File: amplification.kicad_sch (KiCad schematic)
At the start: 34 parts, among them Q1 PNP, Q10 PNP, Q11 NPN, Q12 NPN, Q13 NPN, Q14 PNP, Q15 NPN, Q16 PNP, Q2 PNP, Q3 NPN, Q4 PNP, Q5 NPN, Q6 PNP, Q7 NPN, Q8 NPN, Q9 PNP

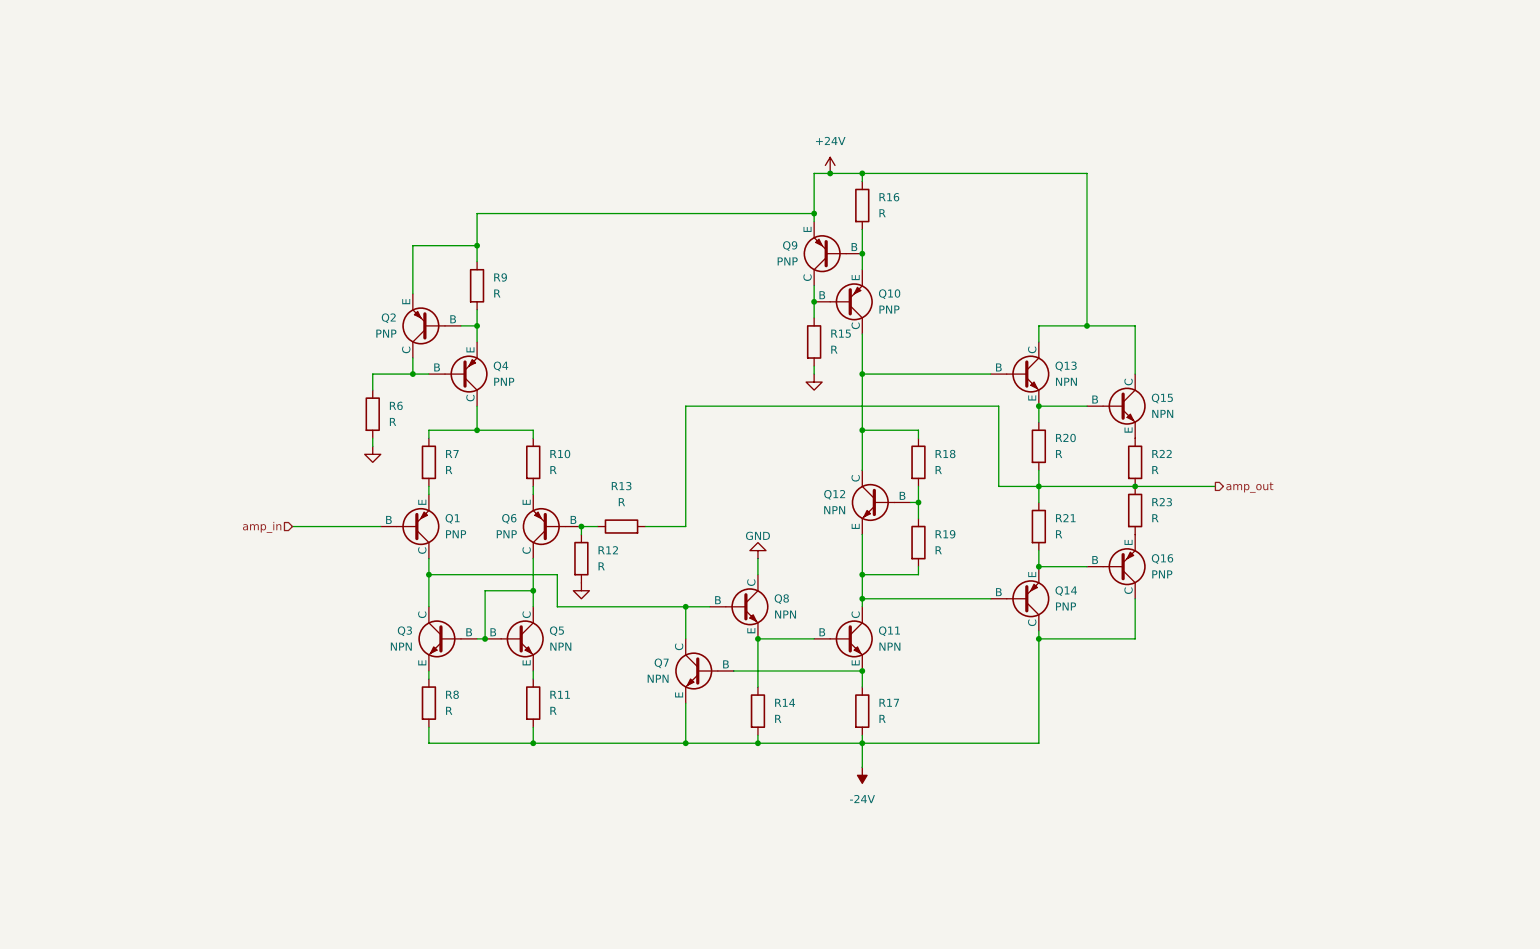
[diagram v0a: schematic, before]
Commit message: organize amp sheet
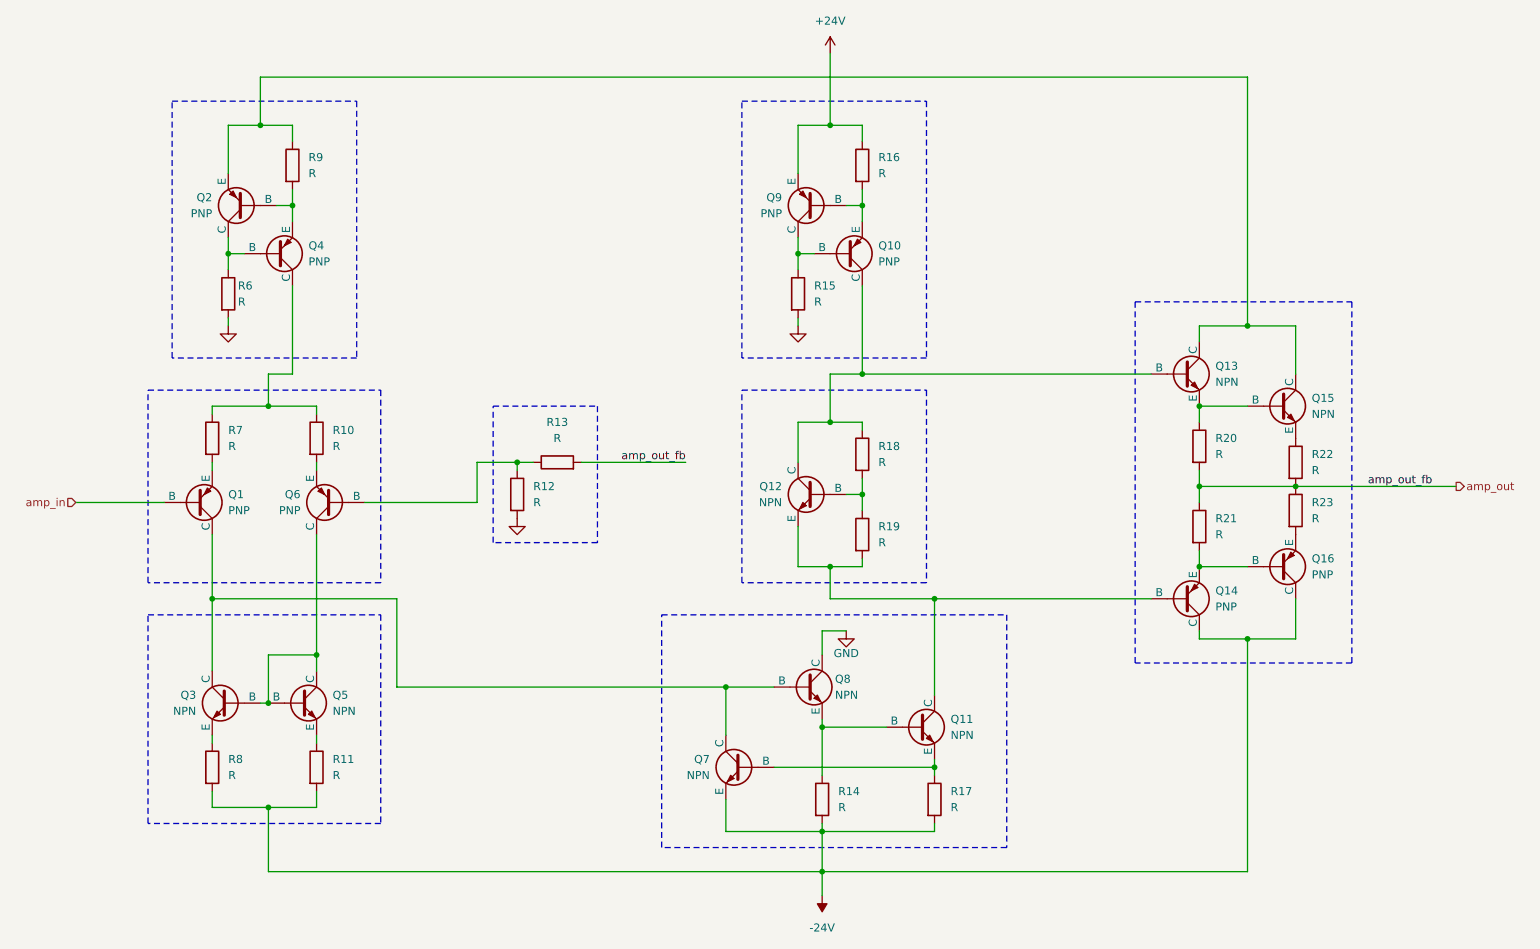
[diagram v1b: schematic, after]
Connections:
- net +24V: no longer Q13.1 (C), Q15.1 (C), Q2.3 (E), R9.1
- new net: Q13.1 (C), Q15.1 (C), Q2.3 (E), R9.1
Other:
- moved on the sheet: Q10, Q11, Q7, Q8, Q9, R14, R15, R16, R17
